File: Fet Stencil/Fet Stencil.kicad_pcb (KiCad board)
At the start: 2 copper layers, 7.4 x 6 mm, 1 part, among them U1 BSC066N06NSATMA1

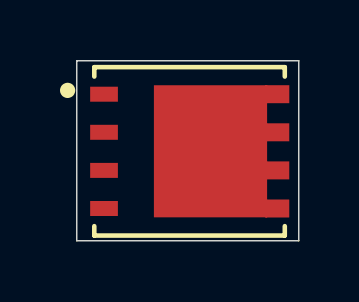
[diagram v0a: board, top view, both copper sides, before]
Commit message: V1 finished. Final touchups to schematic planned
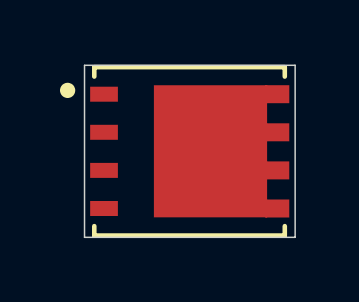
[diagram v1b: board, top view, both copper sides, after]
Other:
- board size 7.4 x 6 mm -> 7 x 5.7 mm
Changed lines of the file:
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@@
 	)
 	(gr_rect
-		(start 129.6 105)
-		(end 137 111)
+		(start 129.859572 105.151698)
+		(end 136.88 110.886181)
 		(stroke
 			(width 0.05)
